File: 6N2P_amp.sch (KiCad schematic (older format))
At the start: 39 parts, among them J1 6.3MMTRSSwitched, U1 ECC83, U2 ECC83

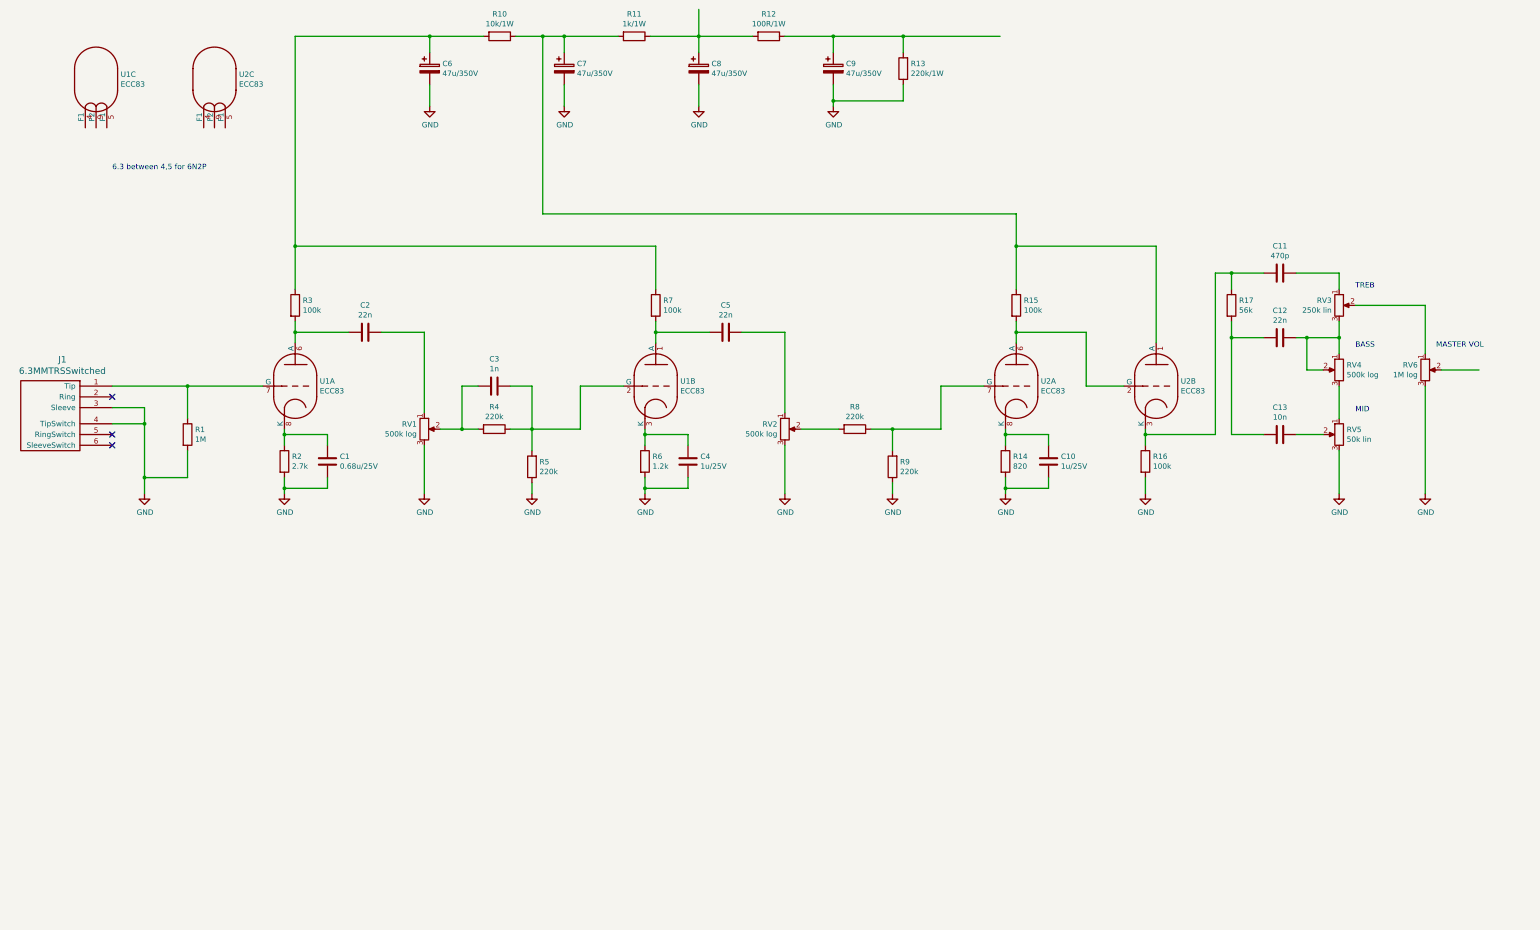
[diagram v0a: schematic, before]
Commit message: snap
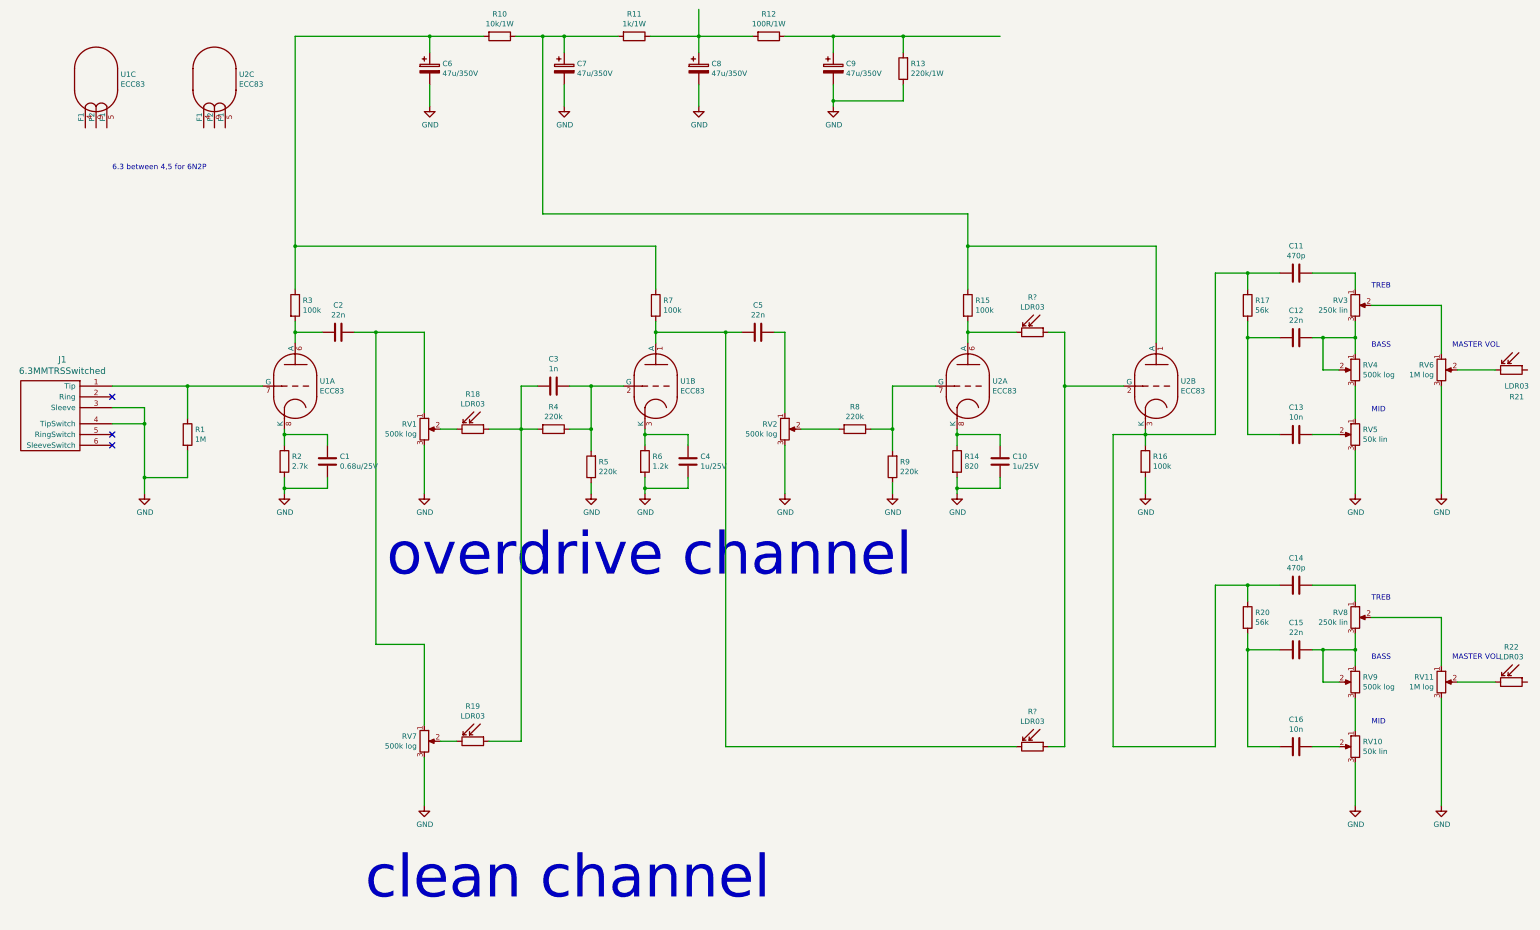
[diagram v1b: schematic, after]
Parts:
- added C14: 470p, Capacitor_THT:C_Rect_L9.0mm_W4.0mm_P7.50mm_MKT, symbol Device:C
- added C15: 22n, Capacitor_THT:C_Rect_L9.0mm_W4.0mm_P7.50mm_MKT, symbol Device:C
- added C16: 10n, Capacitor_THT:C_Rect_L9.0mm_W4.0mm_P7.50mm_MKT, symbol Device:C
- added R18, R19, R21, R22, R? (x2): LDR03, OptoDevice:R_LDR_10x8.5mm_P7.6mm_Vertical, symbol Sensor_Optical:LDR03
- added R20: 56k, Resistor_THT:R_Axial_DIN0207_L6.3mm_D2.5mm_P10.16mm_Horizontal, symbol Device:R
- added RV10: 50k lin, symbol Device:R_POT
- added RV11: 1M log, symbol Device:R_POT
- added RV7, RV9: 500k log, symbol Device:R_POT
- added RV8: 250k lin, symbol Device:R_POT
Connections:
- net GND: now also RV10.3, RV11.3, RV7.3
- net at C5.2, R7.2, U1.1 (A): now also R?.2
- net at C2.1, RV1.1: now also RV7.1
- net at C3.2, R4.2: now also R18.1, R19.1; no longer RV1.2
- net at R15.2, U2.6 (A): now also R?.2; no longer U2.2 (G)
- net at C11.2, R16.1, R17.1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: now also C14.2, R20.1
- net at RV6.2: now also R21.2
- new net: R18.2, RV1.2
- new net: R?.1, R?.1, U2.2 (G)
- new net: R19.2, RV7.2
- new net: RV10.1, RV9.3
- new net: C16.1, RV10.2
- new net: C15.1, RV8.3, RV9.1, RV9.2
- new net: C15.2, C16.2, R20.2
- new net: C14.1, RV8.1
- new net: RV11.1, RV8.2
- new net: R22.2, RV11.2
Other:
- note added: "clean channel"
- note added: "overdrive channel"
- moved on the sheet: C10, C11, C12, C13, C2, C3, C5, R14, R15, R17, R4, R5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
